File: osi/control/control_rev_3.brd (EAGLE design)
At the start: 25.4 x 25.4 mm, 13 parts, among them IC1 UA7805CKCS, IC2 MCP1702

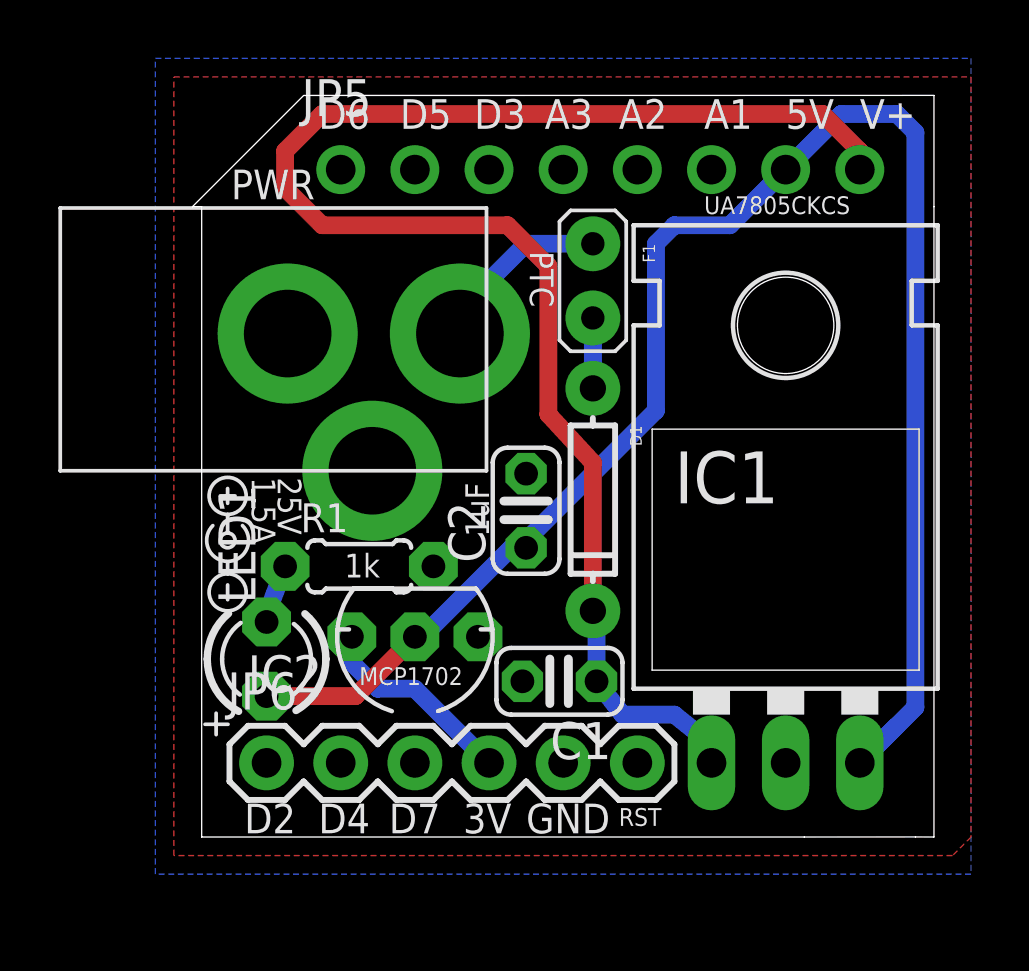
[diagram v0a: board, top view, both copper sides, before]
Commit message: furby board production
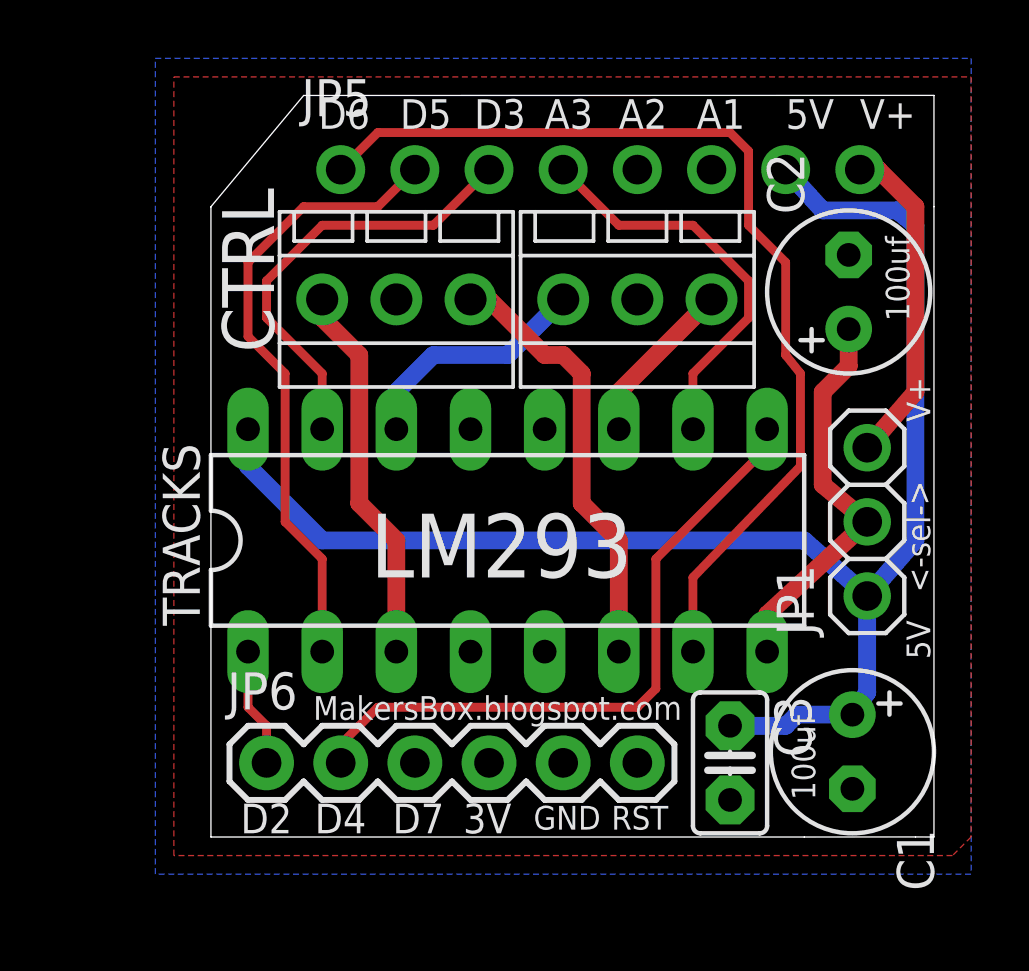
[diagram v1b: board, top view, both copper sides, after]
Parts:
- removed D1: (no value), SparkFun:DIODE-1N4148
- removed F1: PTCPTH, SparkFun_mod:PTC
- removed IC1: UA7805CKCS, SparkFun:TO-220-ALT
- removed IC2: MCP1702, adafruit:TO92-INLINE
- removed LED1: (no value), adafruit:LED3MM
- removed R1: 1k, adafruit:0204/5
- removed U$1: 2.1MMJACKTHM, adafruit:PJ-102A
- removed U$2: (no value), DC_SYM:DC_POS_CTR
- removed U$3: (no value), DC_SYM:DC_POS_CTR-BOTTOM
- added C3: 0.1uF, rcl-ez:C025-025X050
- added JP1: (no value), adafruit_mod:1X03
- added MTR1, MTR2: TERMINAL, _my-parts:TERMINAL_3
- added TRACKS: L293D, texas:DIL16
- C1: value 0.33uF -> 100uF/16V; device adafruit:C025-024X044 -> rcl-ez:E2,5-6
- C2: value 1uF -> 100uF/16V; device adafruit:C025-024X044 -> rcl-ez:E2,5-6
- moved C2 13.4 mm to (22.5, 18.7)
- moved C1 10.3 mm to (22.6, 2.92), turned to 270 degrees
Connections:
- net D10 renamed D7-D13
- net D11 renamed A1-A6
- net D12 renamed A2-A7
- removed net A0: JP5.2
- removed net A1: JP5.1
- removed net A2: JP6.1
- removed net A3: JP6.2
- removed net A7: JP5.3
- removed net D13: JP5.4
- new net A3-A0: JP5.4, TRACKS.10
- new net D2-D8: JP6.1, TRACKS.1
- new net D3-D9: JP5.3, TRACKS.15
- new net D4-D12: JP6.2, TRACKS.9
- new net D5-D10: JP5.2, TRACKS.2
- new net D6-D11: JP5.1, TRACKS.7
- new net N$4: MTR2.P$3, TRACKS.11
- new net N$8: C2.+, JP1.2, TRACKS.8
- net +3V3: no longer IC2.3
- net +5V: now also C1.+, C3.1, JP1.1, TRACKS.16; no longer C2.1, IC1.OUT, IC2.2, LED1.A
- net GND: now also C1.-, C2.-, C3.2, MTR1.P$2, MTR2.P$2, TRACKS.12, TRACKS.13, TRACKS.4, TRACKS.5; no longer C1.2, C2.2, IC1.GND, IC2.1, R1.2, U$1.RING
- net N$1: now also MTR1.P$1, TRACKS.3; no longer F1.P$1, U$1.TIP
- net N$2: now also MTR2.P$1, TRACKS.14; no longer LED1.K, R1.1
- net N$3: now also MTR1.P$3, TRACKS.6; no longer D1.A, F1.P$2
- net V+: now also JP1.3; no longer C1.1, D1.C, IC1.IN
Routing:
- net V+: track 53.1 -> 11.3 mm
- net D6-D11: track 0.00 -> 34.1 mm
- net D4-D12: track 0.00 -> 22.7 mm
- net D5-D10: track 0.00 -> 21.4 mm
- net D3-D9: track 0.00 -> 15.1 mm
- net A3-A0: track 0.00 -> 13.8 mm
- net N$8: track 0.00 -> 13.6 mm
- net N$3: track 2.41 -> 14.9 mm
- net +3V3: track 7.07 -> 0.00 mm
- net +5V: track 58.4 -> 51.4 mm
- net N$1: track 6.30 -> 13.1 mm
- net N$2: track 2.02 -> 8.30 mm
- net N$4: track 0.00 -> 5.76 mm
- net D2-D8: track 0.00 -> 4.07 mm
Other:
- board size 25.4 x 25.4 mm -> 24.8 x 25.4 mm
- board text added: "100uf"
- board text added: "<-sel->"
- board text added: "Apr 12"
- board text added: "CNTRL"
- board text added: "CTRL"
- board text added: "LM293"
- board text removed: "1.5A"
- board text removed: "1k"
- board text removed: "1uF"
- board text removed: "25V"
- board text removed: "3V: 0.25A"
- board text removed: "5V: 1.5A"
- board text removed: "7-25 VDC"
- board text removed: "Apr 13"
- board text removed: "MCP1702"
- board text removed: "PTC"
- board text removed: "PWR"
- board text removed: "UA7805CKCS"
